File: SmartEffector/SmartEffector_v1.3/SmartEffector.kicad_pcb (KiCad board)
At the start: 2 copper layers, 88.4 x 76.6 mm, 57 parts, among them M1 FID, M10 M_2.9mm, M11 M_2.9mm, M13 Ziptie, M15 OSHW_Logo, M16 12mm, M2 FID, M3 M_3.8mm, M4 M_3.8mm, M5 M_3.8mm, M6 M_3.8mm, M7 M_3.8mm, M8 M_3.8mm, M9 M_2.9mm, M97 M2_1.4mm, M98 M2_1.4mm, M99 M2_1.4mm, P2 PROG, P3 INPUT2, P4 HEATER, P5 TEMP, P7 Print Fan, P8 Input 1, P9 Hotend Fan, U1 LDK130M08, U2 ATTINY45, U3 MCP6286

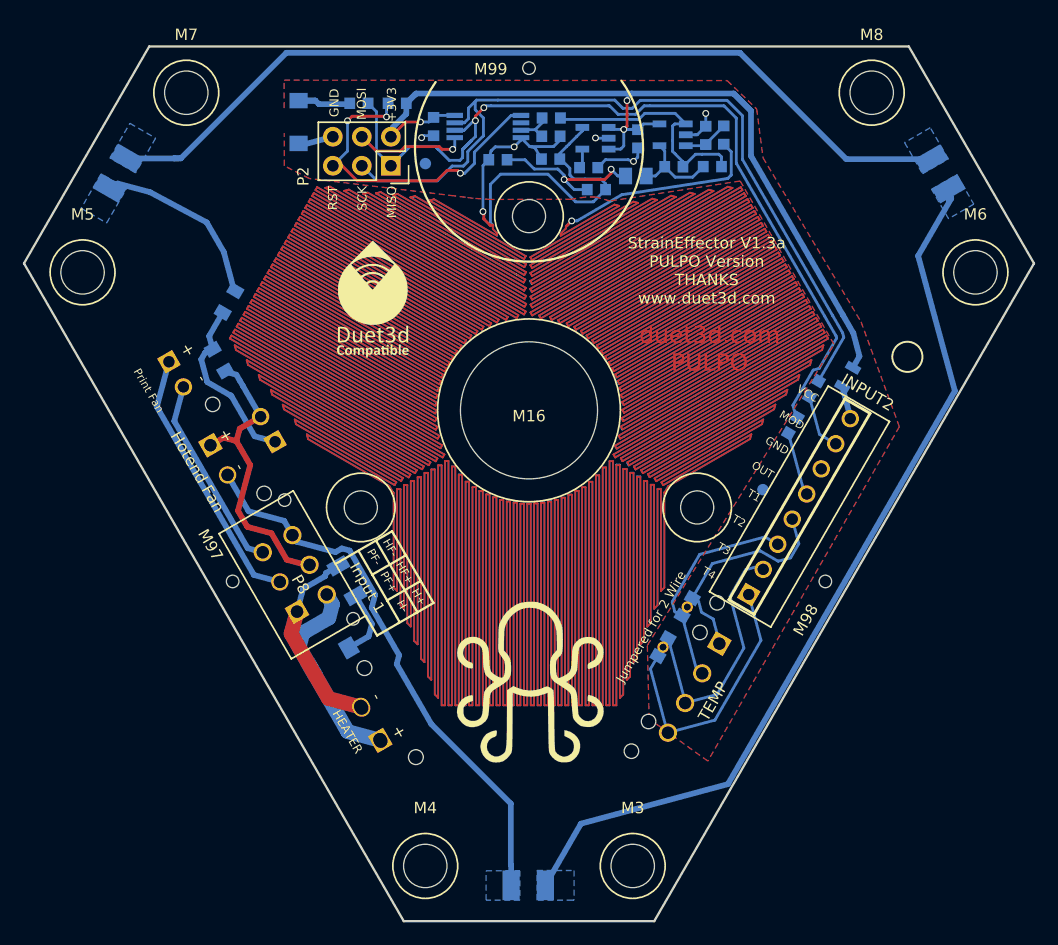
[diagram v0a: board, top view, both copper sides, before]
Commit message: charlio modification, gerbers and autogenerated BOM list
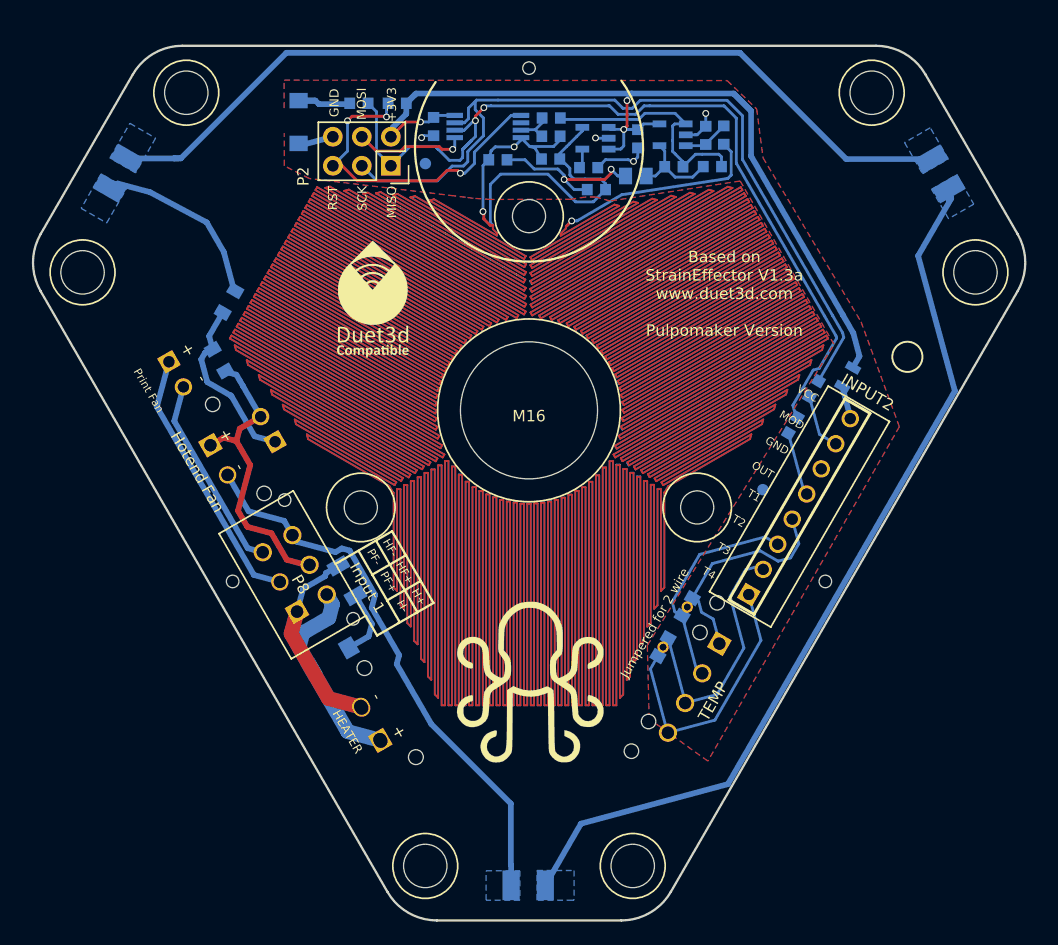
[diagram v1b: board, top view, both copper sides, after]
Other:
- board size 88.4 x 76.6 mm -> 86.9 x 76.6 mm
- board text added: "Based on StrainEffector V1.3a www.duet3d.com Pulpomaker Version"
- board text added: "David Carlos Sergio Santi Raúl Xavi Oriol Victor Javier"
- board text added: "Jumpered for 2 wire"
- board text removed: "Jumpered for 2 Wire"
- board text removed: "StrainEffector V1.3a PULPO Version THANKS www.duet3d.com"
- board text removed: "duet3d.com PULPO"
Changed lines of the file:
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@@
-(kicad_pcb (version 20171130) (host pcbnew 5.0.0+dfsg1-2)
+(kicad_pcb (version 20171130) (host pcbnew "(5.0.0)")
   (general
     (thickness 1.6)
-    (drawings 77)
+    (drawings 82)
     (tracks 1429)
     (zones 0)
@@
     (0 F.Cu signal)
     (31 B.Cu signal)
-    (32 B.Adhes user)
-    (33 F.Adhes user)
-    (34 B.Paste user)
-    (35 F.Paste user)
+    (32 B.Adhes user hide)
+    (33 F.Adhes user hide)
+    (34 B.Paste user hide)
+    (35 F.Paste user hide)
     (36 B.SilkS user)
     (37 F.SilkS user)
     (38 B.Mask user)
     (39 F.Mask user)
-    (40 Dwgs.User user)
-    (41 Cmts.User user)
-    (42 Eco1.User user)
-    (43 Eco2.User user)
+    (40 Dwgs.User user hide)
+    (41 Cmts.User user hide)
+    (42 Eco1.User user hide)
+    (43 Eco2.User user hide)
     (44 Edge.Cuts user)
-    (45 Margin user)
-    (46 B.CrtYd user)
-    (47 F.CrtYd user)
-    (48 B.Fab user)
-    (49 F.Fab user)
+    (45 Margin user hide)
+    (46 B.CrtYd user hide)
+    (47 F.CrtYd user hide)
+    (48 B.Fab user hide)
+    (49 F.Fab user hide)
   )
   (setup
@@
   (module Wire_Pads:M4_3.8 locked (layer F.Cu)
     (at 45.106803 113.838022)
-    (fp_text reference M5 (at 0 -5.08) (layer F.SilkS)
+    (fp_text reference M5 (at 0 -5.08) (layer F.SilkS) hide
       (effects (font (size 1 1) (thickness 0.15)))
     )
@@
   (module Wire_Pads:M4_3.8 locked (layer F.Cu)
     (at 54.186944 98.110756)
-    (fp_text reference M7 (at 0 -5.08) (layer F.SilkS)
+    (fp_text reference M7 (at 4.302525 -2.218279) (layer F.SilkS) hide
       (effects (font (size 1 1) (thickness 0.15)))
     )
@@
   (module Wire_Pads:M4_3.8 (layer F.Cu)
     (at 114.186946 98.110757)
-    (fp_text reference M8 (at 0 -5.08) (layer F.SilkS)
+    (fp_text reference M8 (at -3.881477 -1.83728) (layer F.SilkS) hide
       (effects (font (size 1 1) (thickness 0.15)))
     )
@@
   (module Wire_Pads:M4_3.8 locked (layer F.Cu)
     (at 123.267079 113.83802)
-    (fp_text reference M6 (at 0 -5.08) (layer F.SilkS)
+    (fp_text reference M6 (at 1.38939 -3.721543) (layer F.SilkS) hide
       (effects (font (size 1 1) (thickness 0.15)))
     )
@@
   (module Wire_Pads:M4_3.8 locked (layer F.Cu)
     (at 93.267087 165.799547)
-    (fp_text reference M3 (at 0 -5.08) (layer F.SilkS)
+    (fp_text reference M3 (at 0 -5.08) (layer F.SilkS) hide
       (effects (font (size 1 1) (thickness 0.15)))
     )
@@
   (module Wire_Pads:M4_3.8 locked (layer F.Cu)
     (at 75.106796 165.799547)
-    (fp_text reference M4 (at 0 -5.08) (layer F.SilkS)
+    (fp_text reference M4 (at 0 -5.08) (layer F.SilkS) hide
       (effects (font (size 1 1) (thickness 0.15)))
     )
@@
   (module Wire_Pads:M2_2.4 (layer F.Cu)
     (at 84.186943 95.960759)
-    (fp_text reference M99 (at -3.348806 0.084343) (layer F.SilkS)
+    (fp_text reference M99 (at -3.348806 0.084343) (layer F.SilkS) hide
       (effects (font (size 1 1) (thickness 0.15)))
     )
@@
   (module Wire_Pads:M2_2.4 (layer F.Cu)
     (at 58.244843 140.893787 120)
-    (fp_text reference M97 (at 3.736499 -0.083013 120) (layer F.SilkS)
+    (fp_text reference M97 (at 3.736499 -0.083013 120) (layer F.SilkS) hide
       (effects (font (size 1 1) (thickness 0.15)))
     )
@@
   (module Wire_Pads:M2_2.4 (layer F.Cu)
     (at 110.129047 140.893789 240)
-    (fp_text reference M98 (at 3.777945 -0.201285 240) (layer F.SilkS)
+    (fp_text reference M98 (at 3.777945 -0.201285 240) (layer F.SilkS) hide
       (effects (font (size 1 1) (thickness 0.15)))
     )
@@
       (effects (font (size 1 1) (thickness 0.15)) (justify mirror))
     )
-    (fp_text user K (at -3.957066 0.991181 240) (layer B.SilkS)
+    (fp_text user K (at -3.957066 0.991181 240) (layer B.SilkS) hide
       (effects (font (size 0.9 0.9) (thickness 0.1)) (justify mirror))
     )
@@
       (effects (font (size 1 1) (thickness 0.15)) (justify mirror))
     )
-    (fp_text user K (at -4.102768 0.812217) (layer B.SilkS)
+    (fp_text user K (at -4.102768 0.812217) (layer B.SilkS) hide
       (effects (font (size 0.9 0.9) (thickness 0.1)) (justify mirror))
     )
@@
       (effects (font (size 1 1) (thickness 0.15)) (justify mirror))
     )
-    (fp_text user K (at -3.41469 0.797969 120) (layer B.SilkS)
+    (fp_text user K (at -3.41469 0.797969 120) (layer B.SilkS) hide
       (effects (font (size 0.9 0.9) (thickness 0.1)) (justify mirror))
     )
@@
       (xy -1.056581 0.682429)) (layer F.SilkS) (width 0.01))
   )
+  (gr_line (start 126.959844 115.486448) (end 96.601596 168.068477) (layer Edge.Cuts) (width 0.2))
+  (gr_arc (start 53.839971 99.003171) (end 53.839971 94.003171) (angle -60) (layer Edge.Cuts) (width 0.2))
+  (gr_arc (start 45.766723 112.986448) (end 41.436596 110.486448) (angle -60) (layer Edge.Cuts) (width 0.2))
+  (gr_line (start 53.839971 94.003171) (end 114.556469 94.003171) (layer Edge.Cuts) (width 0.2))
+  (gr_arc (start 114.556469 99.003171) (end 118.886596 96.503171) (angle -60) (layer Edge.Cuts) (width 0.2))
+  (gr_line (start 118.886596 96.503171) (end 126.959844 110.486448) (layer Edge.Cuts) (width 0.2))
+  (gr_arc (start 122.629717 112.986448) (end 126.959844 115.486448) (angle -60) (layer Edge.Cuts) (width 0.2))
+  (gr_arc (start 92.271469 165.568477) (end 92.271469 170.568477) (angle -60) (layer Edge.Cuts) (width 0.2))
+  (gr_arc (start 76.124971 165.568477) (end 71.794844 168.068477) (angle -60) (layer Edge.Cuts) (width 0.2))
+  (gr_line (start 71.794844 168.068477) (end 41.436596 115.486448) (layer Edge.Cuts) (width 0.2))
+  (gr_line (start 41.436596 110.486448) (end 49.509844 96.503171) (layer Edge.Cuts) (width 0.2))
+  (gr_line (start 92.271469 170.568477) (end 76.124971 170.568477) (layer Edge.Cuts) (width 0.2))
   (gr_text T2 (at 102.562039 135.614841 -30) (layer F.SilkS)
     (effects (font (size 0.7 0.7) (thickness 0.08)))
@@
   )
   (gr_arc (start 84.186942 102.916111) (end 92.272014 97.055601) (angle 251) (layer F.SilkS) (width 0.2))
-  (gr_text "Jumpered for 2 Wire" (at 94.875525 144.858812 60) (layer F.SilkS)
+  (gr_text "Jumpered for 2 wire" (at 95.192469 144.533477 60) (layer F.SilkS)
     (effects (font (size 0.8 0.8) (thickness 0.1)))
   )
@@
     (effects (font (size 0.8 0.8) (thickness 0.1)) (justify right))
   )
-  (gr_text "duet3d.com\nPULPO" (at 99.994702 120.529389) (layer F.Mask)
-    (effects (font (size 1.5 1.5) (thickness 0.26)))
-  )
-  (gr_text "duet3d.com\nPULPO" (at 99.997469 120.530477) (layer F.Cu)
-    (effects (font (size 1.5 1.5) (thickness 0.3)))
+  (gr_text "David\nCarlos\nSergio\nSanti\nRaúl\nXavi\nOriol\nVictor\nJavier" (at 98.367469 118.879477) (layer Dwgs.User)
+    (effects (font (size 1.5 1.5) (thickness 0.26)) (justify mirror))
   )
   (gr_text "RST\n\nSCK\n\nMISO" (at 69.593453 106.259225 90) (layer F.SilkS)
@@
     (effects (font (size 1 1) (thickness 0.1)))
   )
-  (gr_text "StrainEffector V1.3a\nPULPO Version\nTHANKS\nwww.duet3d.com" (at 99.744701 113.68939) (layer F.SilkS)
+  (gr_text "Based on\nStrainEffector V1.3a\nwww.duet3d.com\n\nPulpomaker Version\n" (at 101.288469 115.704477) (layer F.SilkS)
     (effects (font (size 1 1) (thickness 0.2)))
   )
-  (gr_line (start 39.979186 113.049393) (end 73.225969 170.634506) (angle 90) (layer Edge.Cuts) (width 0.2))
-  (gr_line (start 50.940158 94.064428) (end 39.979183 113.049396) (angle 90) (layer Edge.Cuts) (width 0.2))
-  (gr_line (start 117.433727 94.064431) (end 50.940159 94.064432) (angle 90) (layer Edge.Cuts) (width 0.2))
-  (gr_line (start 128.394701 113.04939) (end 117.433728 94.064424) (angle 90) (layer Edge.Cuts) (width 0.2))
-  (gr_line (start 95.14792 170.634512) (end 128.394704 113.049389) (angle 90) (layer Edge.Cuts) (width 0.2))
-  (gr_line (start 95.14792 170.634512) (end 73.225967 170.634514) (angle 90) (layer Edge.Cuts) (width 0.2))
   (segment (start 72.096943 101.966108) (end 72.096943 101.601112) (width 0.5) (layer B.Cu) (net 1))
   (segment (start 112.534436 122.190205) (end 113.118868 121.177945) (width 0.5) (layer B.Cu) (net 1))
